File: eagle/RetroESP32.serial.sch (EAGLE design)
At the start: 70 parts, among them J1 AUDIO_JACK_3.5MM_KIT, J5 503182-1852_503182-1852, J6 USB4110-GF-A_REVB, Q3 DMG3415U-7, Q4 mmbt2222, Q5 mmbt2222, U1 ESP32-WROVER, U3 XC6210B332MR-G, U4 MCP73832T-2ACI/OT, U6 LM4875, X2 53261-02, X3 53261-02

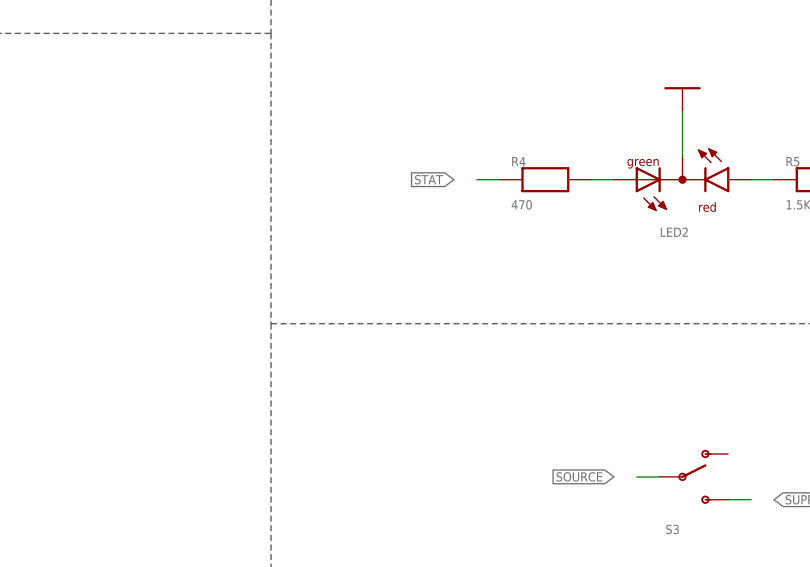
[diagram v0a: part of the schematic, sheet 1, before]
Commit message: feat: released X
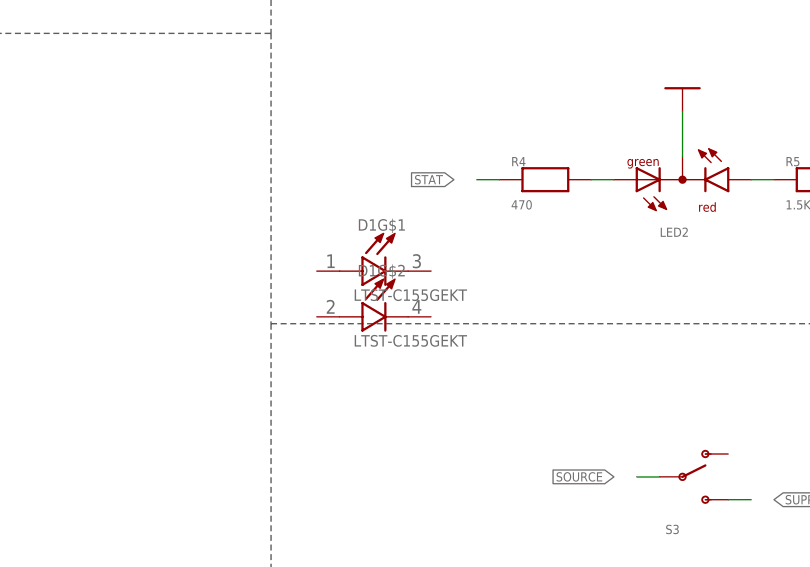
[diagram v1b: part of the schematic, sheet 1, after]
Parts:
- added D1: LTST-C155GEKT, LTST-C155GEKT:LTST-C155GEKT
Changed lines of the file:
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@@
 <attribute name="MPN" value="0532614002"/>
 </part>
+<part name="D1" library="LTST-C155GEKT" deviceset="LTST-C155GEKT" device=""/>
 </parts>
 <sheets>
@@
 <attribute name="MPN" x="132.08" y="53.34" size="1.778" layer="96" display="off"/>
 </instance>
+<instance part="D1" gate="G$1" x="114.3" y="43.18" smashed="yes">
+<attribute name="NAME" x="111.2012" y="47.6758" size="1.27" layer="95"/>
+<attribute name="VALUE" x="110.744" y="39.878" size="1.27" layer="96"/>
+</instance>
+<instance part="D1" gate="G$2" x="114.3" y="38.1" smashed="yes">
+<attribute name="NAME" x="111.2012" y="42.5958" size="1.27" layer="95"/>
+<attribute name="VALUE" x="110.744" y="34.798" size="1.27" layer="96"/>
+</instance>
 </instances>

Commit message: update: BOM for X
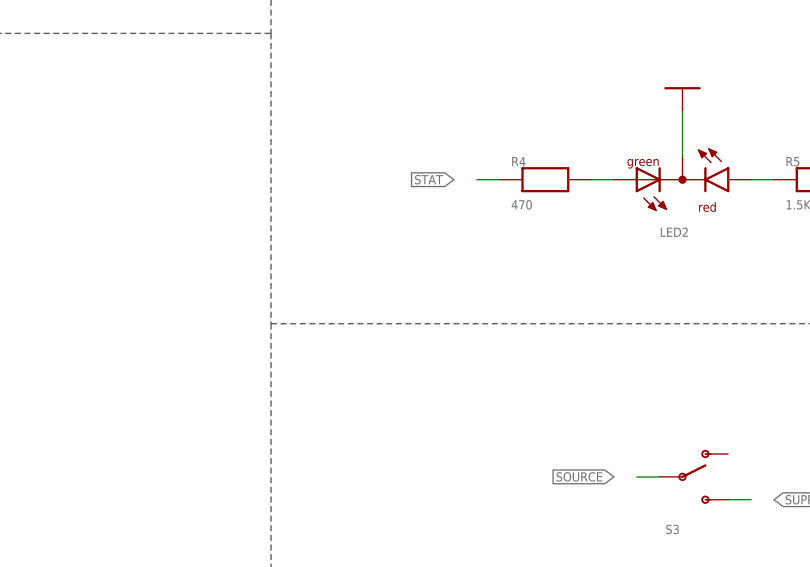
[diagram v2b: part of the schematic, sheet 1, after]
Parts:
- removed D1: LTST-C155GEKT, LTST-C155GEKT:LTST-C155GEKT
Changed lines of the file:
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@@
 <attribute name="MPN" value="0532614002"/>
 </part>
-<part name="D1" library="LTST-C155GEKT" deviceset="LTST-C155GEKT" device=""/>
 </parts>
 <sheets>
@@
 <attribute name="MPN" x="132.08" y="53.34" size="1.778" layer="96" display="off"/>
 </instance>
-<instance part="D1" gate="G$1" x="114.3" y="43.18" smashed="yes">
-<attribute name="NAME" x="111.2012" y="47.6758" size="1.27" layer="95"/>
-<attribute name="VALUE" x="110.744" y="39.878" size="1.27" layer="96"/>
-</instance>
-<instance part="D1" gate="G$2" x="114.3" y="38.1" smashed="yes">
-<attribute name="NAME" x="111.2012" y="42.5958" size="1.27" layer="95"/>
-<attribute name="VALUE" x="110.744" y="34.798" size="1.27" layer="96"/>
-</instance>
 </instances>
